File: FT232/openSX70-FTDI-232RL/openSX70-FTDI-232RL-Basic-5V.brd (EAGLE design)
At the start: 27.9 x 17.3 mm, 13 parts, among them J1 687106183722, U1 FT232RLSSOP

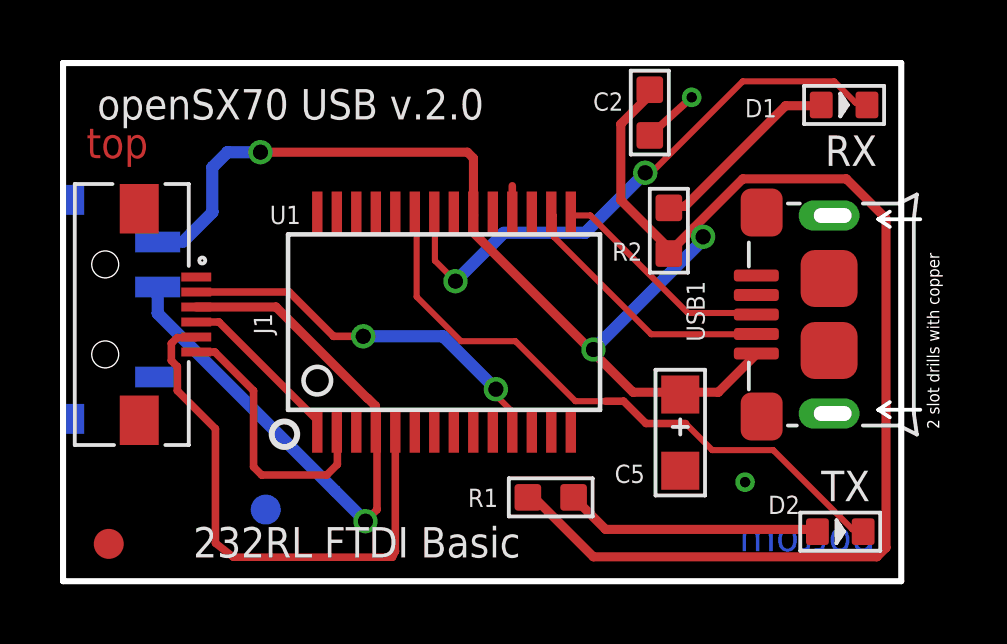
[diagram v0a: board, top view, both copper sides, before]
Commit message: Fixes to power.
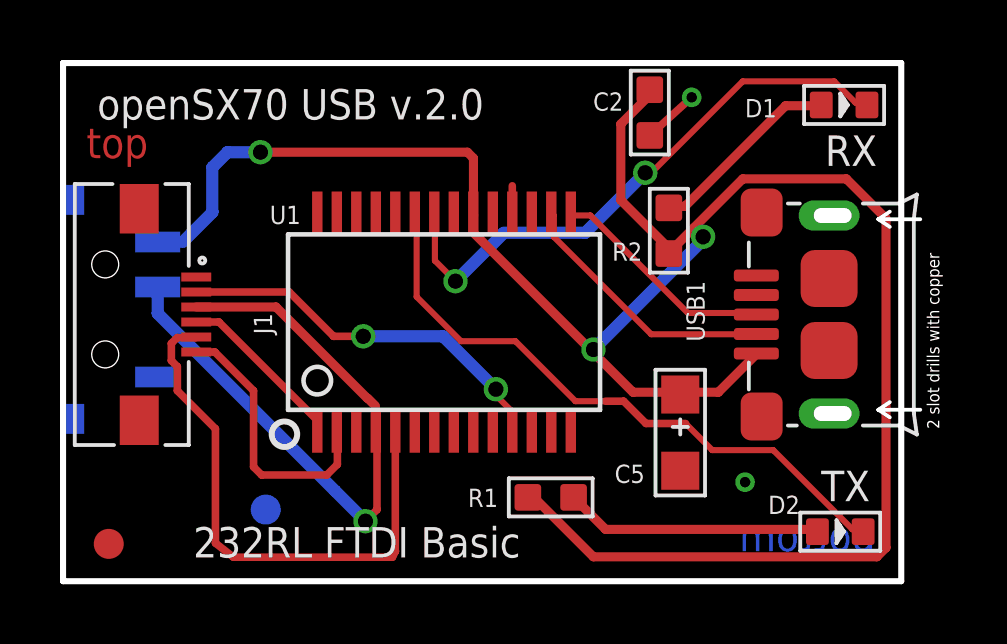
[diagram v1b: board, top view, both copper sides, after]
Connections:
- new net N$4: U1.20, U1.4
- net 5V: no longer U1.20
- net POWER: no longer U1.4
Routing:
- net POWER: track 22.1 -> 21.2 mm
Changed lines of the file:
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@@
 <?xml version="1.0" encoding="utf-8"?>
 <!DOCTYPE eagle SYSTEM "eagle.dtd">
-<eagle version="9.1.0">
+<eagle version="9.0.0">
 <drawing>
 <settings>
@@
 <param name="checkStop" value="0"/>
 <param name="checkValues" value="0"/>
-<param name="checkNames" value="1"/>
-<param name="checkWireStubs" value="1"/>
-<param name="checkPolygonWidth" value="0"/>
 <param name="useDiameter" value="13"/>
 <param name="maxErrors" value="50"/>
@@
 </signal>
 <signal name="POWER">
-<contactref element="U1" pad="4"/>
 <contactref element="J1" pad="3"/>
 <wire x1="5.3848" y1="4.9784" x2="5.3848" y2="4.2672" width="0.2032" layer="1"/>
-<wire x1="5.3848" y1="4.9784" x2="5.345" y2="4.98" width="0.2032" layer="1"/>
 <wire x1="-0.64" y1="9.14" x2="2.02" y2="9.14" width="0.3048" layer="1"/>
 <wire x1="5.064" y1="6.096" x2="2.02" y2="9.14" width="0.3048" layer="1"/>
-<wire x1="5.345" y1="4.98" x2="5.334" y2="5.842" width="0.3048" layer="1"/>
 <wire x1="5.334" y1="5.842" x2="5.08" y2="6.096" width="0.3048" layer="1"/>
 <wire x1="5.08" y1="6.096" x2="5.064" y2="6.096" width="0.254" layer="1"/>
@@
 <wire x1="5.3848" y1="2.3848" x2="5.3848" y2="4.2672" width="0.254" layer="1"/>
 <wire x1="-1.925" y1="8.925" x2="4" y2="3" width="0.4064" layer="16"/>
+<wire x1="5.3848" y1="4.9784" x2="5.334" y2="5.842" width="0" layer="19" extent="1-1"/>
 </signal>
 <signal name="5V">
-<contactref element="U1" pad="20"/>
 <contactref element="C5" pad="+"/>
 <contactref element="C2" pad="1"/>
@@
 <wire x1="12.5476" y1="7.6708" x2="8.636" y2="11.5824" width="0.3048" layer="1"/>
 <wire x1="15.4432" y1="6.2992" x2="13.9192" y2="6.2992" width="0.3048" layer="1"/>
-<wire x1="8.636" y1="12.192" x2="8.595" y2="12.292" width="0.2032" layer="1"/>
 <wire x1="15.4432" y1="6.2992" x2="15.494" y2="6.223" width="0.2032" layer="1"/>
 <wire x1="10.668" y1="2.7432" x2="10.4648" y2="2.7432" width="0.2032" layer="1"/>
@@
 <wire x1="18.03" y1="8.24" x2="18.0212" y2="8.2312" width="0.2032" layer="1"/>
 </signal>
+<signal name="N$4">
+<contactref element="U1" pad="4"/>
+<contactref element="U1" pad="20"/>
+<wire x1="5.345" y1="4.98" x2="8.595" y2="12.292" width="0" layer="19" extent="1-1"/>
+</signal>
 </signals>
-<mfgpreviewcolors>
-<mfgpreviewcolor name="soldermaskcolor" color="0xC8008000"/>
-<mfgpreviewcolor name="silkscreencolor" color="0xFFFEFEFE"/>
-<mfgpreviewcolor name="backgroundcolor" color="0xFF282828"/>
-<mfgpreviewcolor name="coppercolor" color="0xFFFFBF00"/>
-<mfgpreviewcolor name="substratecolor" color="0xFF786E46"/>
-</mfgpreviewcolors>
 <errors>
 </errors>
